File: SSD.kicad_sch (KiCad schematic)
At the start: 9 parts, among them J8 1935174, K1 EE2-12NUH, Q6 BSP296NH6327XTSA1

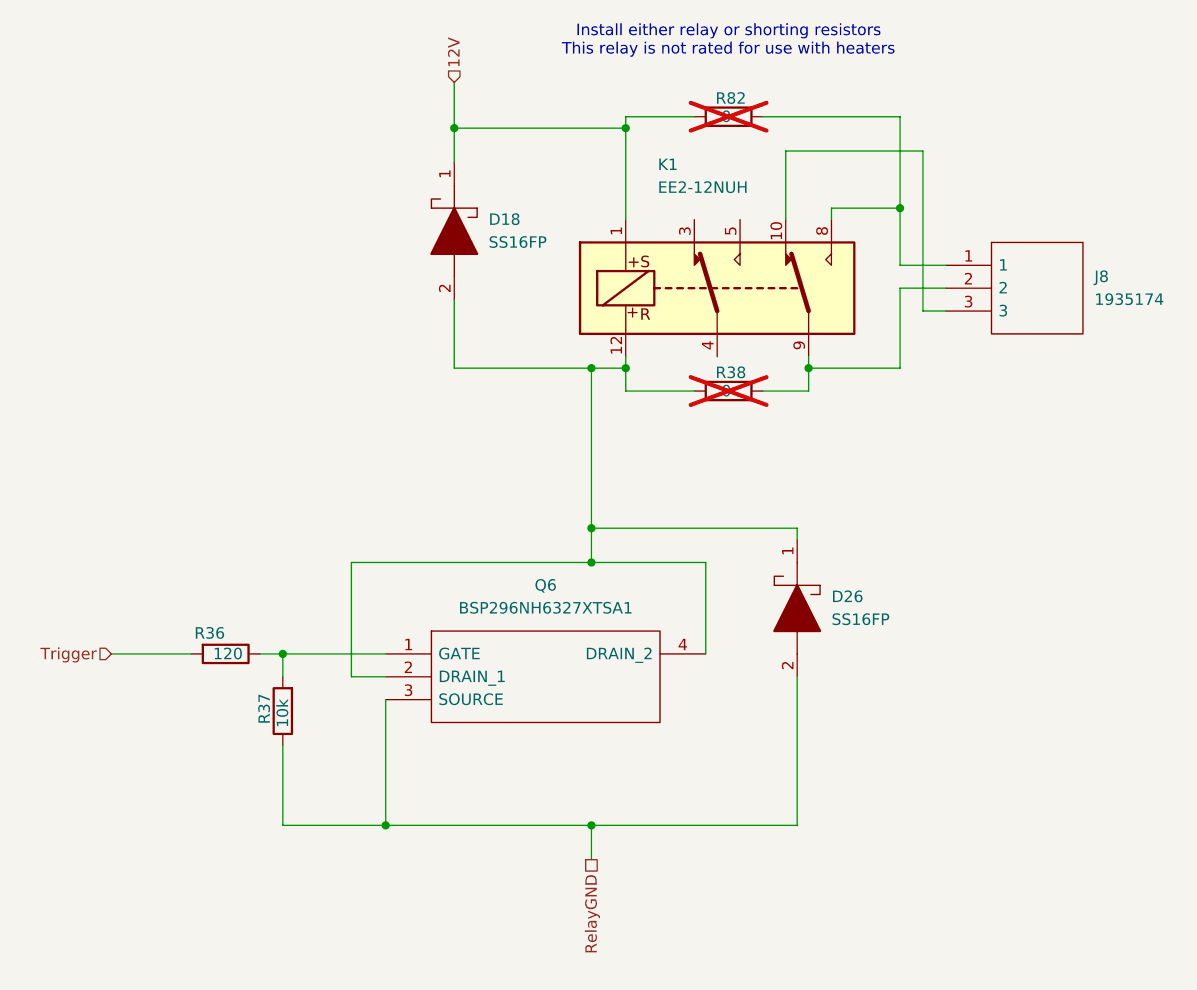
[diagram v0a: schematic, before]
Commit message: sch looks prety good
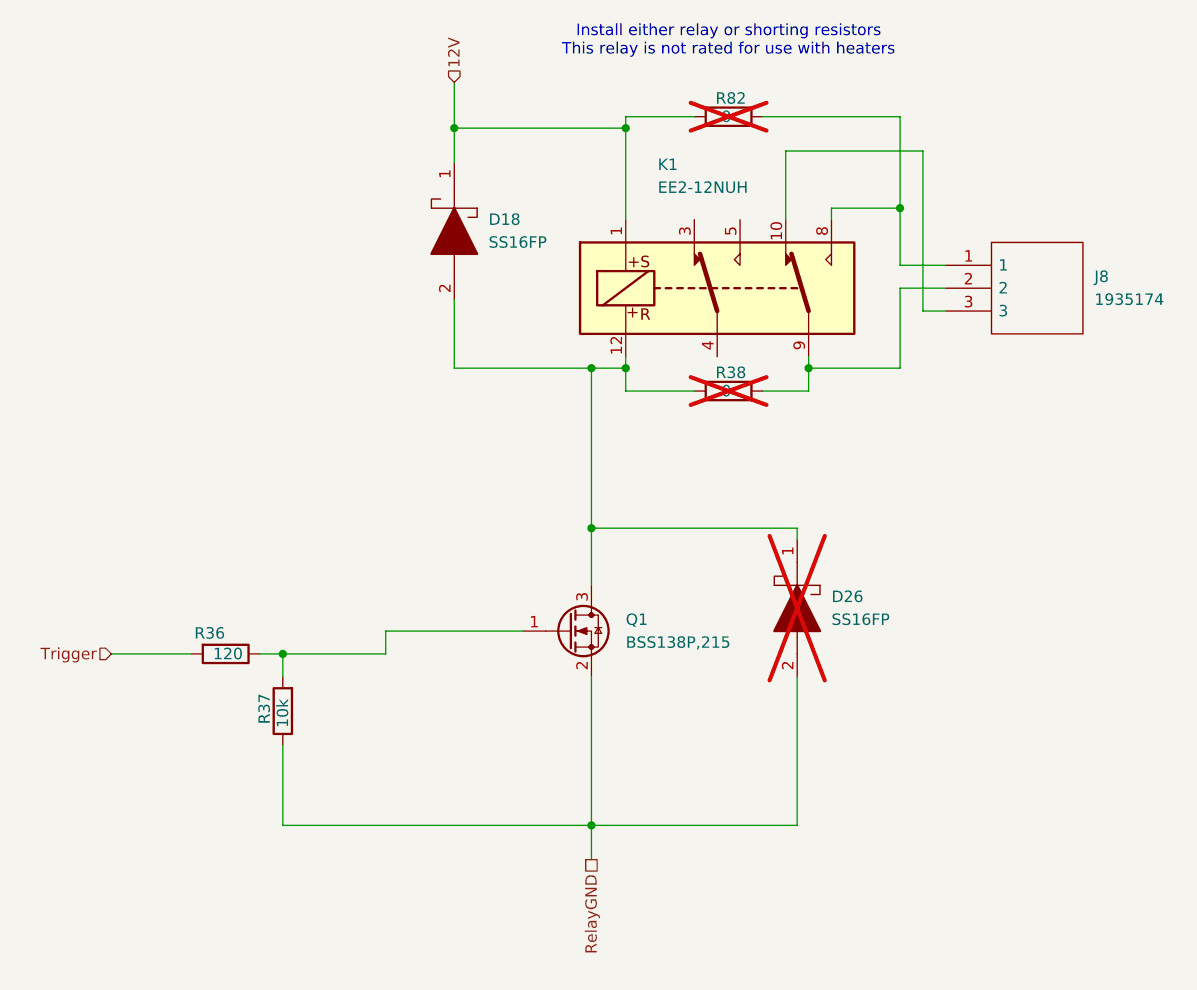
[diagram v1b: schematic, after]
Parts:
- removed Q6: BSP296NH6327XTSA1, SamacSys_Parts:SOT230P700X170-4N, symbol SamacSys_Parts:BSP296NH6327XTSA1
- added Q1: BSS138P,215, Package_TO_SOT_SMD:SOT-23, symbol Transistor_FET:BSS138
- D26: now not fitted
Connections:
- net RelayGND: now also Q1.2 (S)
- net at R36.1, R37.2: now also Q1.1 (G)
- net at D18.2, D26.1, K1.12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: now also Q1.3 (D)
